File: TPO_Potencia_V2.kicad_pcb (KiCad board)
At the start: 2 copper layers, 110 x 71 mm, 30 parts, among them J1 Entrada_Alterna, J2 Entrada 220V Trafo, J3 Salida 12V alt, J4 Entrada_DC, J5 Conn_02x03_Odd_Even, SW1 SW_DIP_x01, U1 SSM3K16FU, U2 IR2153, U3 STP12N50M2, U4 STP12N50M2, U5 DB153

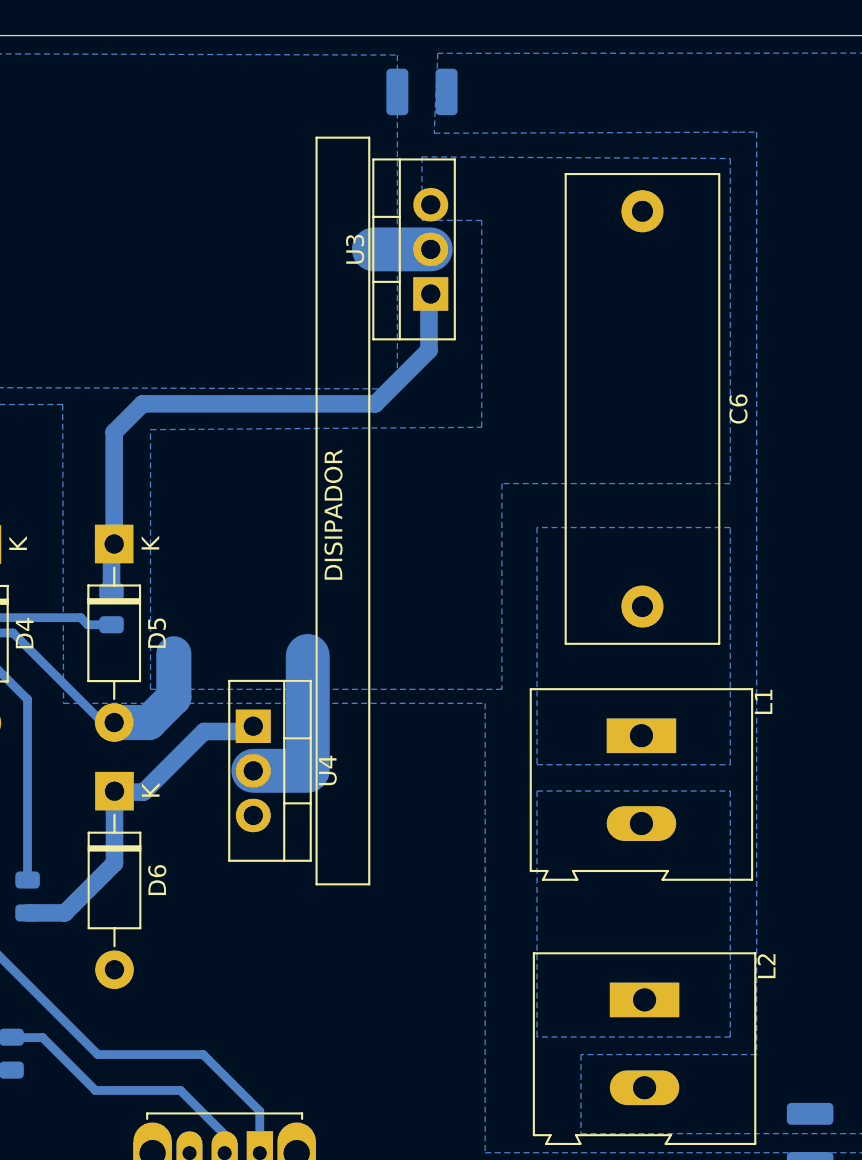
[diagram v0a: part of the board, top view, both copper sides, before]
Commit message: PCB terminado
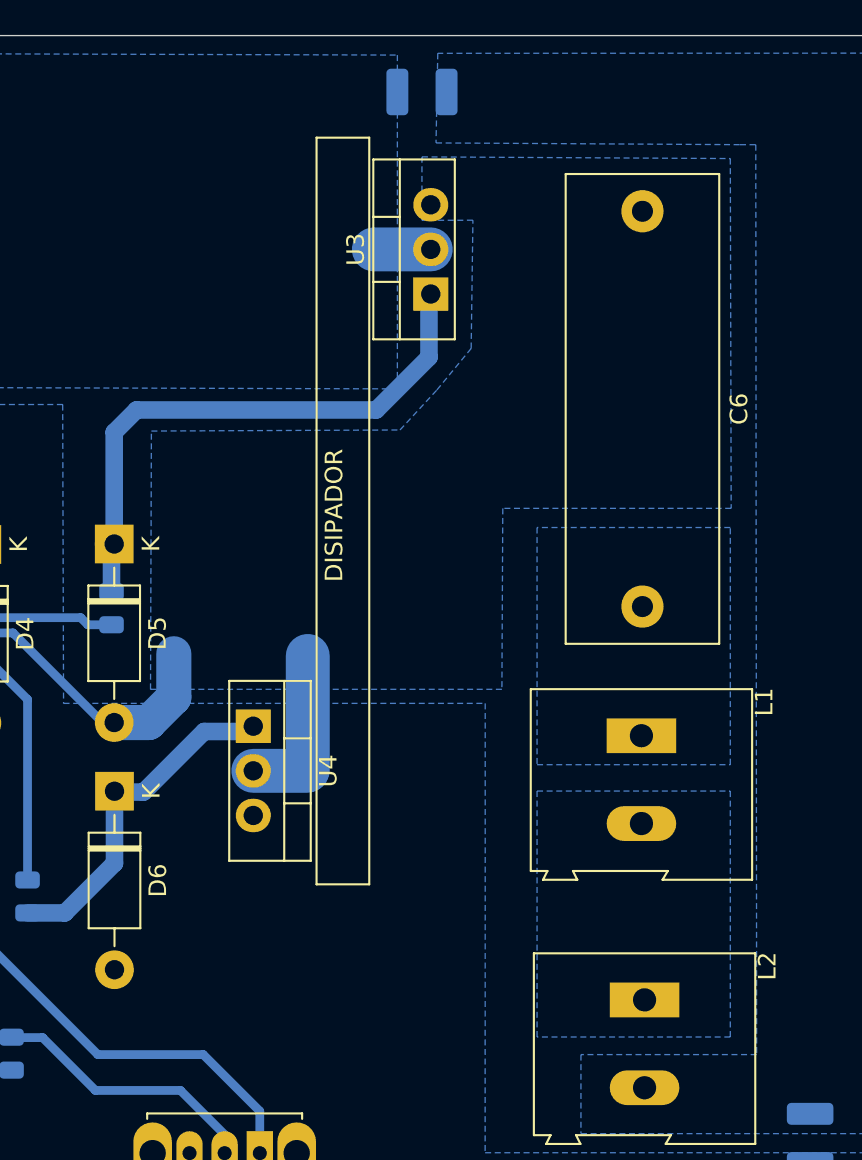
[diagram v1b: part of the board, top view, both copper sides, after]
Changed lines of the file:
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@@
     (user_trace_width 5)
     (trace_clearance 0.2)
-    (zone_clearance 0.508)
+    (zone_clearance 1)
     (zone_45_only no)
     (trace_min 0.2)
@@
   (segment (start 147.33 81.5876) (end 146.8728 81.1304) (width 1) (layer B.Cu) (net 13))
   (segment (start 147.33 83.772) (end 147.33 81.5876) (width 1) (layer B.Cu) (net 13))
-  (segment (start 165.4 70.1) (end 165.4 66.9) (width 1) (layer B.Cu) (net 13))
-  (segment (start 162.348 73.152) (end 165.4 70.1) (width 1) (layer B.Cu) (net 13))
-  (segment (start 149.098 73.152) (end 162.348 73.152) (width 1) (layer B.Cu) (net 13))
+  (segment (start 148.75 73.5) (end 162.4 73.5) (width 1) (layer B.Cu) (net 13))
   (segment (start 147.4824 81.1304) (end 147.4824 74.7676) (width 1) (layer B.Cu) (net 13))
-  (segment (start 147.4824 74.7676) (end 149.098 73.152) (width 1) (layer B.Cu) (net 13))
+  (segment (start 165.4 70.5) (end 165.4 66.9) (width 1) (layer B.Cu) (net 13))
+  (segment (start 162.4 73.5) (end 165.4 70.5) (width 1) (layer B.Cu) (net 13))
+  (segment (start 147.4824 74.7676) (end 148.75 73.5) (width 1) (layer B.Cu) (net 13))
   (segment (start 152.6 91.8) (end 155.5 91.8) (width 1) (layer B.Cu) (net 14))
   (segment (start 147.55 95.25) (end 149.15 95.25) (width 1) (layer B.Cu) (net 14))
@@
   (segment (start 142.55 89.9775) (end 139.71 87.1375) (width 0.5) (layer B.Cu) (net 24))
   (zone (net 7) (net_name /V_DC_Pulsante) (layer B.Cu) (hatch edge 0.508)
-    (connect_pads yes (clearance 0.508))
-    (min_thickness 0.254)
+    (connect_pads yes (clearance 1))
+    (min_thickness 0.5)
     (fill yes (arc_segments 32) (thermal_gap 0.508) (thermal_bridge_width 0.508))
     (polygon
@@
   )
   (zone (net 6) (net_name "Net-(C4-Pad2)") (layer B.Cu) (hatch edge 0.508)
-    (connect_pads yes (clearance 0.508))
-    (min_thickness 0.254)
+    (connect_pads yes (clearance 1))
+    (min_thickness 0.5)
     (fill yes (arc_segments 32) (thermal_gap 0.508) (thermal_bridge_width 0.508))
     (polygon
       (pts
-        (xy 165.9 53.2) (xy 165.7 57.75) (xy 183.05 57.69) (xy 184.05 57.69) (xy 184.05 110.19)
+        (xy 165.9 53.2) (xy 165.8 58.3) (xy 183.1 58.4) (xy 184 58.4) (xy 184.05 110.19)
         (xy 174.05 110.19) (xy 174.05 114.69) (xy 191.05 114.69) (xy 190.8 53.19)
       )
@@
   )
   (zone (net 8) (net_name "Net-(C6-Pad2)") (layer B.Cu) (hatch edge 0.508)
-    (connect_pads yes (clearance 0.508))
-    (min_thickness 0.254)
+    (connect_pads yes (clearance 1))
+    (min_thickness 0.5)
     (fill yes (arc_segments 32) (thermal_gap 0.508) (thermal_bridge_width 0.508))
     (polygon
@@
   )
   (zone (net 19) (net_name "Net-(L1-Pad2)") (layer B.Cu) (hatch edge 0.508)
-    (connect_pads yes (clearance 0.508))
-    (min_thickness 0.254)
+    (connect_pads yes (clearance 1))
+    (min_thickness 0.5)
     (fill yes (arc_segments 32) (thermal_gap 0.508) (thermal_bridge_width 0.508))
     (polygon
@@
   )
   (zone (net 5) (net_name "Net-(C3-Pad2)") (layer B.Cu) (hatch edge 0.508)
-    (connect_pads yes (clearance 0.508))
-    (min_thickness 0.254)
+    (connect_pads yes (clearance 1))
+    (min_thickness 0.5)
     (fill yes (arc_segments 32) (thermal_gap 0.508) (thermal_bridge_width 0.508))
     (polygon
       (pts
-        (xy 182.55 77.69) (xy 169.55 77.69) (xy 169.55 89.4) (xy 149.55 89.4) (xy 149.55 74.62)
-        (xy 168.4 74.486) (xy 168.4 62.714) (xy 165 62.705) (xy 165 59.095) (xy 182.55 59.19)
+        (xy 182.6 79.1) (xy 169.6 79.1) (xy 169.55 89.4) (xy 149.55 89.4) (xy 149.6 74.7)
+        (xy 163.749535 74.638741) (xy 165.850465 72.361259) (xy 167.8 70) (xy 167.9 62.7) (xy 165 62.705)
+        (xy 165 59.095) (xy 182.55 59.19)
       )
     )
